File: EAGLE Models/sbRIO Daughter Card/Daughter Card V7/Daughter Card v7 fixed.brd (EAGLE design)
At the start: 136.7 x 102.9 mm, 92 parts, among them IC1 BTS716G, IC10 MIC5225-3.3YM5-TR, IC11 MIC5225-3.3YM5-TR, IC12 MIC5225-3.3YM5-TR, IC2 BTS716G, IC3 BTS716G, IC4 ADXL345, IC5 L3G4200D, IC8 MIC5225-3.3YM5-TR, IC9 MIC5225-3.3YM5-TR, K1 HE3621A1250_SPST, K2 HE3621A1250_SPST, K3 HE3621A1250_SPST, K4 HE3621A1250_SPST, K5 HE3621A1250_SPST, K6 HE3621A1250_SPST, Q1 MMBT4403-7-F, Q2 MMBT4403-7-F, Q3 MMBT4401-7-F, Q4 MMBT4401-7-F, U1 DMN3404L-7

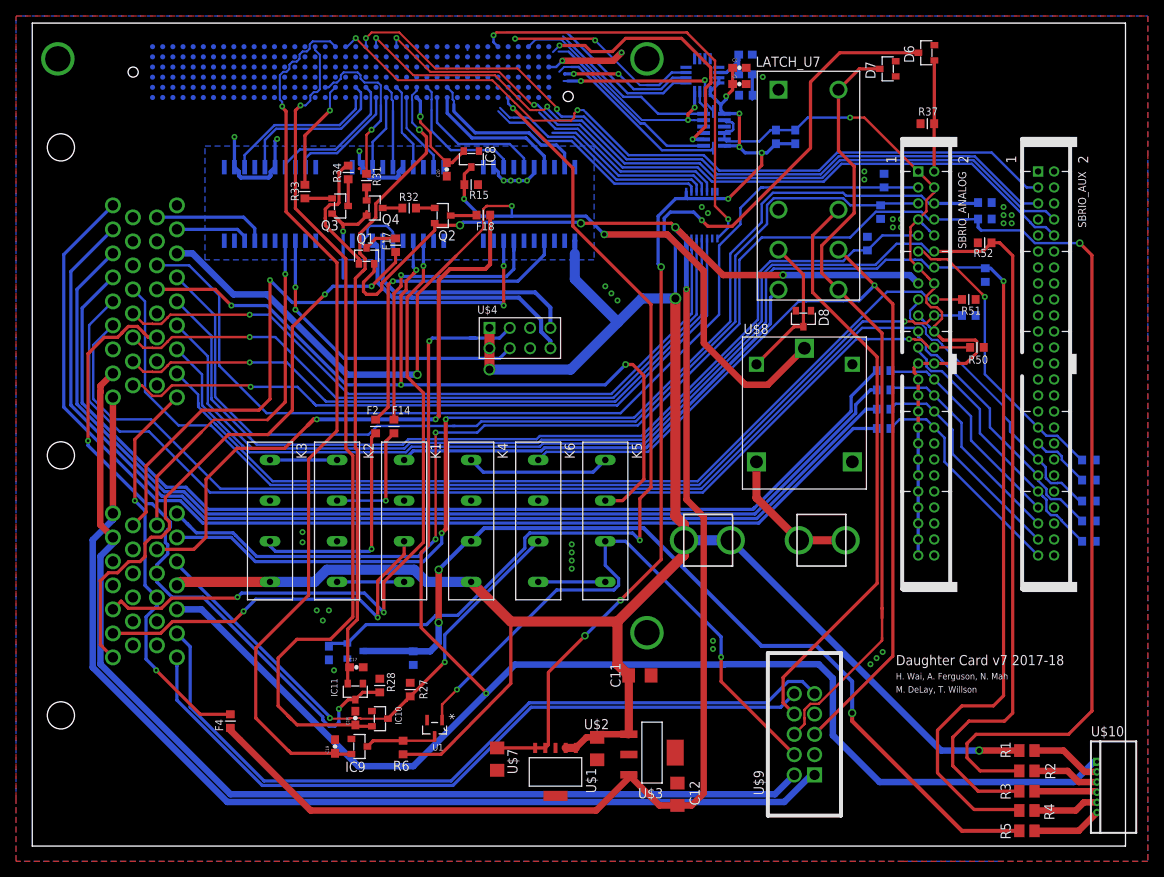
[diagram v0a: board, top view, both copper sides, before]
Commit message: continued fixing dfm issues
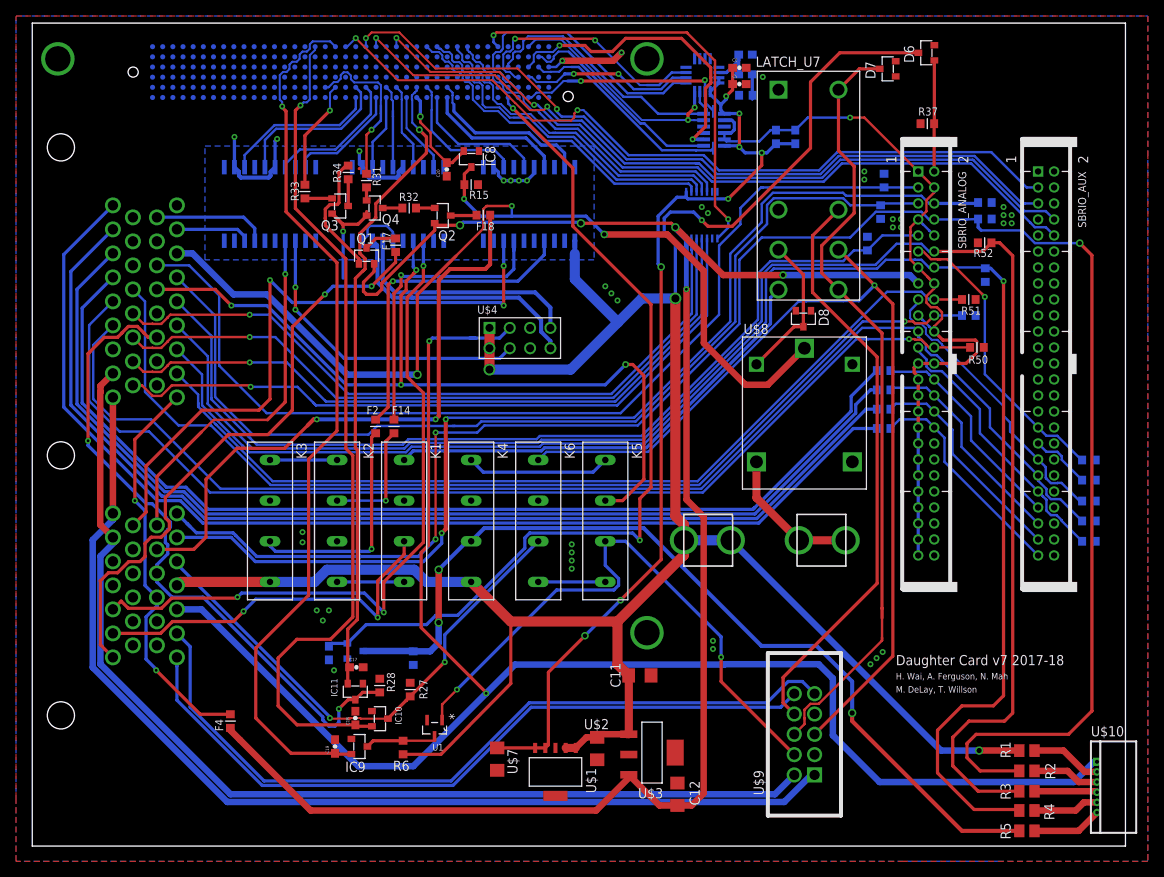
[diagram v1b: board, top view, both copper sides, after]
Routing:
- net DIO86: track 22.3 -> 41.5 mm
- net DIO88: track 28.7 -> 42.9 mm
- net DIO85: track 26.2 -> 40.0 mm
- net DIO87: track 29.5 -> 43.1 mm
- net DIO32: track 26.1 -> 36.1 mm
- net DIO18: track 24.9 -> 34.5 mm
- net DIO65: track 24.5 -> 31.5 mm
- net DIO0: track 22.1 -> 27.3 mm
- net DIO64: track 16.6 -> 21.8 mm
- net DIO17: track 33.9 -> 38.2 mm
- net DIO48: track 36.1 -> 39.6 mm
- net DIO16: track 24.0 -> 26.9 mm
- net DIO95: track 107.2 -> 105.7 mm
- net DIO45: track 20.7 -> 21.8 mm
- net DIO41: track 10.3 -> 11.1 mm

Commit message: finished making all gerbers. Ready to send out
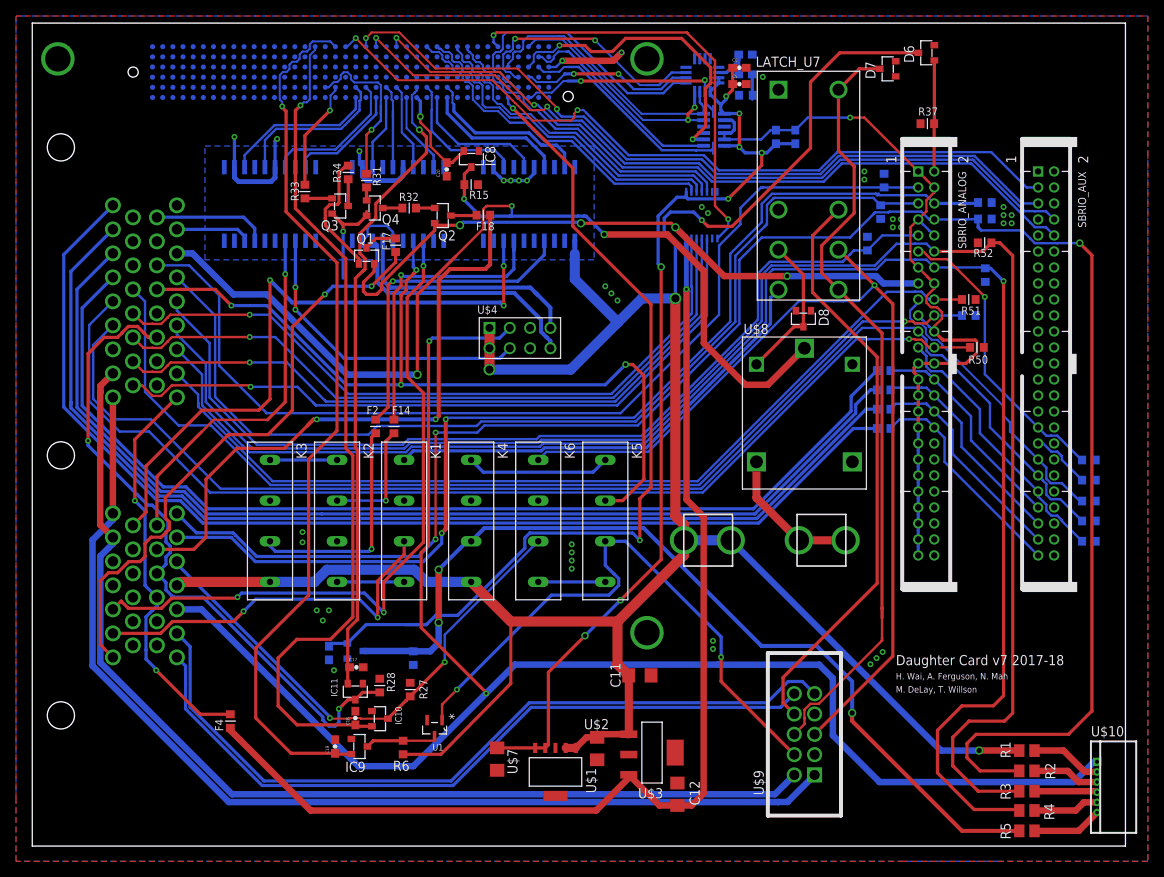
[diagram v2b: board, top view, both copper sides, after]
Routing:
- net DIO48: track 39.6 -> 26.7 mm
- net DIO1: track 109.2 -> 111.9 mm
- net GND: track 54.6 -> 56.9 mm
- net BMS_CAN_H: track 92.8 -> 91.7 mm
- net LATCH_SW_OUT: track 119.5 -> 118.6 mm
- net SIGNAL_GND: track 199.0 -> 198.3 mm
- net DIO92: track 97.1 -> 96.4 mm
- net N$9: track 136.6 -> 137.2 mm
- net DIO42: track 17.3 -> 17.8 mm
